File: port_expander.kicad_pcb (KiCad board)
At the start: 2 copper layers, 101.6 x 50.8 mm, 17 parts, among them J0 Conn_01x08_Male, J1 Conn_01x08_Male, J10 Conn_01x06_Male, J2 Conn_01x08_Male, J3 Conn_01x08_Male, J4 Conn_01x08_Male, J5 Conn_01x08_Male, J6 Conn_01x08_Male, J7 Conn_01x08_Male, J8 Conn_01x08_Male, J9 Conn_01x08_Male, U1 74LS30

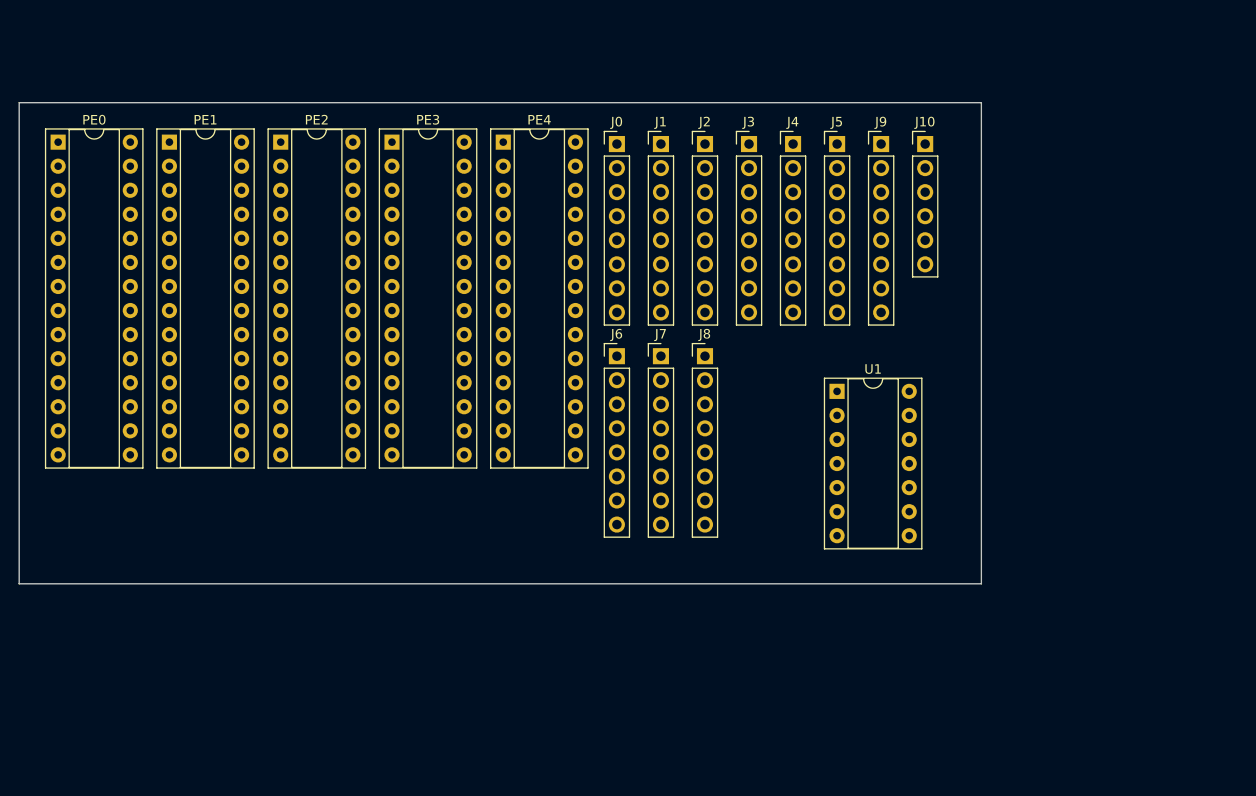
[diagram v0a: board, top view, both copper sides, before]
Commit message: first pcb iteration
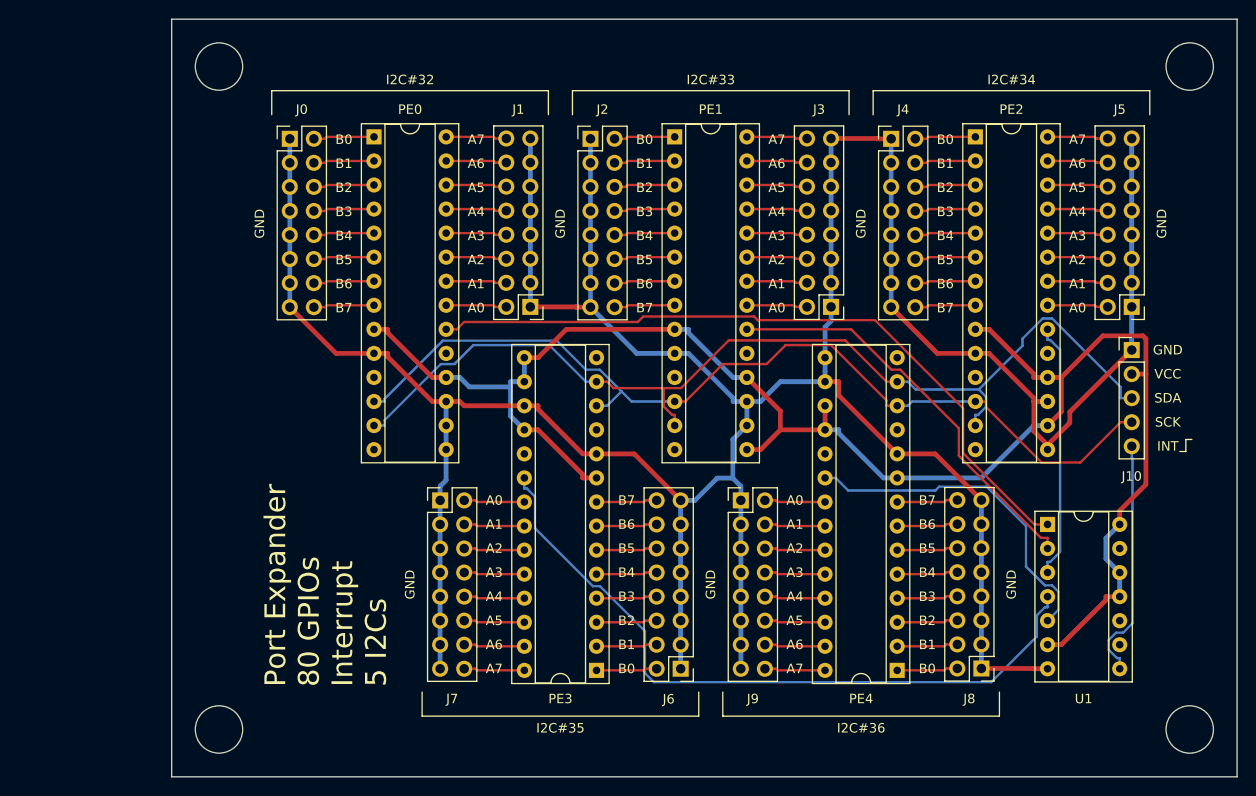
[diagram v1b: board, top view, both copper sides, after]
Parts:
- J0, J1, J2, J3, J4, J5, J6, J7, J8, J9: value Conn_01x08_Male -> Conn_02x08_Male; footprint Connector_PinHeader_2.54mm:PinHeader_1x08_P2.54mm_Vertical -> Connector_PinHeader_2.54mm:PinHeader_2x08_P2.54mm_Vertical
- J10: value Conn_01x06_Male -> Conn_01x05_Male; footprint Connector_PinHeader_2.54mm:PinHeader_1x06_P2.54mm_Vertical -> Connector_PinHeader_2.54mm:PinHeader_1x05_P2.54mm_Vertical
- moved PE2 73.4 mm to (189.9, 87.4)
- moved PE4 69.6 mm to (181.6, 143.8), turned to 180 degrees
- moved PE3 59.8 mm to (149.9, 143.8), turned to 180 degrees
- moved PE1 53.4 mm to (158.1, 87.4)
- moved J8 44.0 mm to (190.5, 143.6), turned to 180 degrees
- moved J9 40.4 mm to (165.1, 125.8)
- moved J5 35.5 mm to (206.4, 105.4), turned to 180 degrees
- moved J0 34.5 mm to (117.5, 87.6)
- moved J6 33.7 mm to (158.8, 143.6), turned to 180 degrees
- moved PE0 33.4 mm to (126.4, 87.4)
- moved J10 30.8 mm to (206.4, 109.9)
- moved J7 27.8 mm to (133.3, 125.8)
- moved U1 26.3 mm to (197.5, 128.3)
- moved J1 22.0 mm to (142.9, 105.4), turned to 180 degrees
- moved J3 19.3 mm to (174.6, 105.4), turned to 180 degrees
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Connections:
- J0 pad 1: Net-(J0-Pad1) -> GND
- J0 pad 3: Net-(J0-Pad3) -> GND
- J0 pad 5: Net-(J0-Pad5) -> GND
- J0 pad 7: Net-(J0-Pad7) -> GND
- J1 pad 1: Net-(J1-Pad1) -> GND
- J1 pad 3: Net-(J1-Pad3) -> GND
- J1 pad 5: Net-(J1-Pad5) -> GND
- J1 pad 7: Net-(J1-Pad7) -> GND
- J2 pad 1: Net-(J2-Pad1) -> GND
- J2 pad 3: Net-(J2-Pad3) -> GND
- J2 pad 5: Net-(J2-Pad5) -> GND
- J2 pad 7: Net-(J2-Pad7) -> GND
- J3 pad 1: Net-(J3-Pad1) -> GND
- J3 pad 3: Net-(J3-Pad3) -> GND
- J3 pad 5: Net-(J3-Pad5) -> GND
- J3 pad 7: Net-(J3-Pad7) -> GND
- J4 pad 1: Net-(J4-Pad1) -> GND
- J4 pad 3: Net-(J4-Pad3) -> GND
- J4 pad 5: Net-(J4-Pad5) -> GND
- J4 pad 7: Net-(J4-Pad7) -> GND
- J5 pad 1: Net-(J5-Pad1) -> GND
- J5 pad 3: Net-(J5-Pad3) -> GND
- J5 pad 5: Net-(J5-Pad5) -> GND
- J5 pad 7: Net-(J5-Pad7) -> GND
- J6 pad 1: Net-(J6-Pad1) -> GND
- J6 pad 3: Net-(J6-Pad3) -> GND
- J6 pad 5: Net-(J6-Pad5) -> GND
- J6 pad 7: Net-(J6-Pad7) -> GND
- J7 pad 1: Net-(J7-Pad1) -> GND
- J7 pad 3: Net-(J7-Pad3) -> GND
- J7 pad 5: Net-(J7-Pad5) -> GND
- J7 pad 7: Net-(J7-Pad7) -> GND
- J8 pad 1: Net-(J8-Pad1) -> GND
- J8 pad 3: Net-(J8-Pad3) -> GND
- J8 pad 5: Net-(J8-Pad5) -> GND
- J8 pad 7: Net-(J8-Pad7) -> GND
- J9 pad 1: Net-(J9-Pad1) -> GND
- J9 pad 3: Net-(J9-Pad3) -> GND
- J9 pad 5: Net-(J9-Pad5) -> GND
- J9 pad 7: Net-(J9-Pad7) -> GND
- PE0 pad 1: Net-(J0-Pad1) -> Net-(J0-Pad2)
- PE0 pad 11: Net-(PE0-Pad11) -> (no net)
- PE0 pad 14: Net-(PE0-Pad14) -> (no net)
- PE0 pad 19: Net-(PE0-Pad19) -> (no net)
- PE0 pad 2: Net-(J0-Pad2) -> Net-(J0-Pad4)
- PE0 pad 21: Net-(J1-Pad1) -> Net-(J1-Pad2)
- PE0 pad 22: Net-(J1-Pad2) -> Net-(J1-Pad4)
- PE0 pad 23: Net-(J1-Pad3) -> Net-(J1-Pad6)
- PE0 pad 24: Net-(J1-Pad4) -> Net-(J1-Pad8)
- PE0 pad 25: Net-(J1-Pad5) -> Net-(J1-Pad10)
- PE0 pad 26: Net-(J1-Pad6) -> Net-(J1-Pad12)
- PE0 pad 27: Net-(J1-Pad7) -> Net-(J1-Pad14)
- PE0 pad 28: Net-(J1-Pad8) -> Net-(J1-Pad16)
- PE0 pad 3: Net-(J0-Pad3) -> Net-(J0-Pad6)
- PE0 pad 4: Net-(J0-Pad4) -> Net-(J0-Pad8)
- PE0 pad 5: Net-(J0-Pad5) -> Net-(J0-Pad10)
- PE0 pad 6: Net-(J0-Pad6) -> Net-(J0-Pad12)
- PE0 pad 7: Net-(J0-Pad7) -> Net-(J0-Pad14)
- PE0 pad 8: Net-(J0-Pad8) -> Net-(J0-Pad16)
- PE1 pad 1: Net-(J2-Pad1) -> Net-(J2-Pad2)
- PE1 pad 11: Net-(PE1-Pad11) -> (no net)
- PE1 pad 14: Net-(PE1-Pad14) -> (no net)
- PE1 pad 19: Net-(PE1-Pad19) -> (no net)
- PE1 pad 2: Net-(J2-Pad2) -> Net-(J2-Pad4)
- PE1 pad 21: Net-(J3-Pad1) -> Net-(J3-Pad2)
- PE1 pad 22: Net-(J3-Pad2) -> Net-(J3-Pad4)
- PE1 pad 23: Net-(J3-Pad3) -> Net-(J3-Pad6)
- PE1 pad 24: Net-(J3-Pad4) -> Net-(J3-Pad8)
- PE1 pad 25: Net-(J3-Pad5) -> Net-(J3-Pad10)
- PE1 pad 26: Net-(J3-Pad6) -> Net-(J3-Pad12)
- PE1 pad 27: Net-(J3-Pad7) -> Net-(J3-Pad14)
- PE1 pad 28: Net-(J3-Pad8) -> Net-(J3-Pad16)
- PE1 pad 3: Net-(J2-Pad3) -> Net-(J2-Pad6)
- PE1 pad 4: Net-(J2-Pad4) -> Net-(J2-Pad8)
- PE1 pad 5: Net-(J2-Pad5) -> Net-(J2-Pad10)
- PE1 pad 6: Net-(J2-Pad6) -> Net-(J2-Pad12)
- PE1 pad 7: Net-(J2-Pad7) -> Net-(J2-Pad14)
- PE1 pad 8: Net-(J2-Pad8) -> Net-(J2-Pad16)
- PE2 pad 1: Net-(J4-Pad1) -> Net-(J4-Pad2)
- PE2 pad 11: Net-(PE2-Pad11) -> (no net)
- PE2 pad 14: Net-(PE2-Pad14) -> (no net)
- PE2 pad 19: Net-(PE2-Pad19) -> (no net)
- PE2 pad 2: Net-(J4-Pad2) -> Net-(J4-Pad4)
- PE2 pad 21: Net-(J5-Pad1) -> Net-(J5-Pad2)
- PE2 pad 22: Net-(J5-Pad2) -> Net-(J5-Pad4)
- PE2 pad 23: Net-(J5-Pad3) -> Net-(J5-Pad6)
- PE2 pad 24: Net-(J5-Pad4) -> Net-(J5-Pad8)
- PE2 pad 25: Net-(J5-Pad5) -> Net-(J5-Pad10)
- PE2 pad 26: Net-(J5-Pad6) -> Net-(J5-Pad12)
- PE2 pad 27: Net-(J5-Pad7) -> Net-(J5-Pad14)
- PE2 pad 28: Net-(J5-Pad8) -> Net-(J5-Pad16)
- PE2 pad 3: Net-(J4-Pad3) -> Net-(J4-Pad6)
- PE2 pad 4: Net-(J4-Pad4) -> Net-(J4-Pad8)
- PE2 pad 5: Net-(J4-Pad5) -> Net-(J4-Pad10)
- PE2 pad 6: Net-(J4-Pad6) -> Net-(J4-Pad12)
- PE2 pad 7: Net-(J4-Pad7) -> Net-(J4-Pad14)
- PE2 pad 8: Net-(J4-Pad8) -> Net-(J4-Pad16)
- PE3 pad 1: Net-(J6-Pad1) -> Net-(J6-Pad2)
- PE3 pad 11: Net-(PE3-Pad11) -> (no net)
- PE3 pad 14: Net-(PE3-Pad14) -> (no net)
- PE3 pad 19: Net-(PE3-Pad19) -> (no net)
- PE3 pad 2: Net-(J6-Pad2) -> Net-(J6-Pad4)
- PE3 pad 21: Net-(J7-Pad1) -> Net-(J7-Pad2)
- PE3 pad 22: Net-(J7-Pad2) -> Net-(J7-Pad4)
- PE3 pad 23: Net-(J7-Pad3) -> Net-(J7-Pad6)
- PE3 pad 24: Net-(J7-Pad4) -> Net-(J7-Pad8)
- PE3 pad 25: Net-(J7-Pad5) -> Net-(J7-Pad10)
- PE3 pad 26: Net-(J7-Pad6) -> Net-(J7-Pad12)
- PE3 pad 27: Net-(J7-Pad7) -> Net-(J7-Pad14)
- PE3 pad 28: Net-(J7-Pad8) -> Net-(J7-Pad16)
- PE3 pad 3: Net-(J6-Pad3) -> Net-(J6-Pad6)
- PE3 pad 4: Net-(J6-Pad4) -> Net-(J6-Pad8)
- PE3 pad 5: Net-(J6-Pad5) -> Net-(J6-Pad10)
- PE3 pad 6: Net-(J6-Pad6) -> Net-(J6-Pad12)
- PE3 pad 7: Net-(J6-Pad7) -> Net-(J6-Pad14)
- PE3 pad 8: Net-(J6-Pad8) -> Net-(J6-Pad16)
- PE4 pad 1: Net-(J8-Pad1) -> Net-(J8-Pad2)
- PE4 pad 11: Net-(PE4-Pad11) -> (no net)
- PE4 pad 14: Net-(PE4-Pad14) -> (no net)
- PE4 pad 19: Net-(PE4-Pad19) -> (no net)
- PE4 pad 2: Net-(J8-Pad2) -> Net-(J8-Pad4)
- PE4 pad 21: Net-(J9-Pad1) -> Net-(J9-Pad2)
- PE4 pad 22: Net-(J9-Pad2) -> Net-(J9-Pad4)
- PE4 pad 23: Net-(J9-Pad3) -> Net-(J9-Pad6)
- PE4 pad 24: Net-(J9-Pad4) -> Net-(J9-Pad8)
- PE4 pad 25: Net-(J9-Pad5) -> Net-(J9-Pad10)
- PE4 pad 26: Net-(J9-Pad6) -> Net-(J9-Pad12)
- PE4 pad 27: Net-(J9-Pad7) -> Net-(J9-Pad14)
- PE4 pad 28: Net-(J9-Pad8) -> Net-(J9-Pad16)
- PE4 pad 3: Net-(J8-Pad3) -> Net-(J8-Pad6)
- PE4 pad 4: Net-(J8-Pad4) -> Net-(J8-Pad8)
- PE4 pad 5: Net-(J8-Pad5) -> Net-(J8-Pad10)
- PE4 pad 6: Net-(J8-Pad6) -> Net-(J8-Pad12)
- PE4 pad 7: Net-(J8-Pad7) -> Net-(J8-Pad14)
- PE4 pad 8: Net-(J8-Pad8) -> Net-(J8-Pad16)
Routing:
- net GND: track 0.00 -> 381.7 mm
- net +3V3: track 0.00 -> 179.5 mm
- net /SDA: track 0.00 -> 107.0 mm
- net /SCK: track 0.00 -> 99.2 mm
- net /INT0: track 0.00 -> 75.9 mm
- net /INT3: track 0.00 -> 75.1 mm
- net /INT1: track 0.00 -> 43.7 mm
- net /INT4: track 0.00 -> 36.0 mm
- net /INT2: track 0.00 -> 27.1 mm
- net /INT: track 0.00 -> 25.7 mm
- net Net-(J4-Pad8): track 0.00 -> 6.43 mm
- net Net-(J4-Pad4): track 0.00 -> 6.43 mm
- net Net-(J4-Pad16): track 0.00 -> 6.43 mm
- net Net-(J4-Pad14): track 0.00 -> 6.43 mm
- net Net-(J4-Pad12): track 0.00 -> 6.43 mm
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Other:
- board size 101.6 x 50.8 mm -> 112.5 x 80 mm
- board text added: "A0"
- board text added: "A1"
- board text added: "A2"
- board text added: "A3"
- board text added: "A4"
- board text added: "A5"
- board text added: "A6"
- board text added: "A7"
- board text added: "B0"
- board text added: "B1"
- board text added: "B2"
- board text added: "B3"
- board text added: "B4"
- board text added: "B5"
- board text added: "B6"
- board text added: "B7"
- board text added: "GND"
- board text added: "I2C#32"
- board text added: "I2C#33"
- board text added: "I2C#34"
- board text added: "I2C#35"
- board text added: "I2C#36"
- board text added: "INT"
- board text added: "Port Expander 80 GPIOs Interrupt 5 I2Cs"
- board text added: "SCK"
- board text added: "SDA"
- board text added: "VCC"
